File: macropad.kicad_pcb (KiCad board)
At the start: 2 copper layers, 78.5 x 59.5 mm, 47 parts, among them J1 DX07S016JA1R1500, SW1 SW_Push, SW10 SW_Push, SW2 SW_Push, SW3 SW_Push, SW5 SW_Push, SW6 SW_Push, SW7 SW_Push, SW8 SW_Push, SW9 SW_Push, U1 ATmega16U2-MU, Y1 16MHz

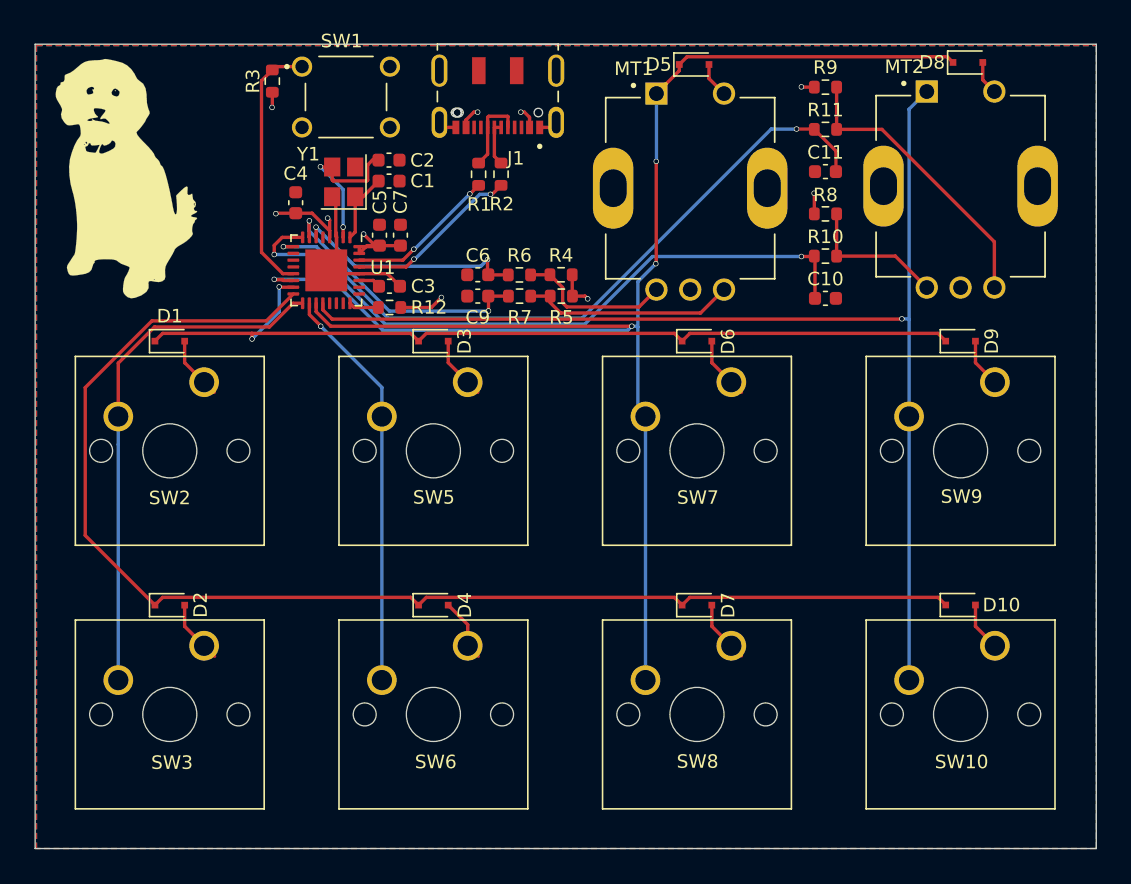
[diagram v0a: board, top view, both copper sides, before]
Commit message: Some aesthetic cleanup
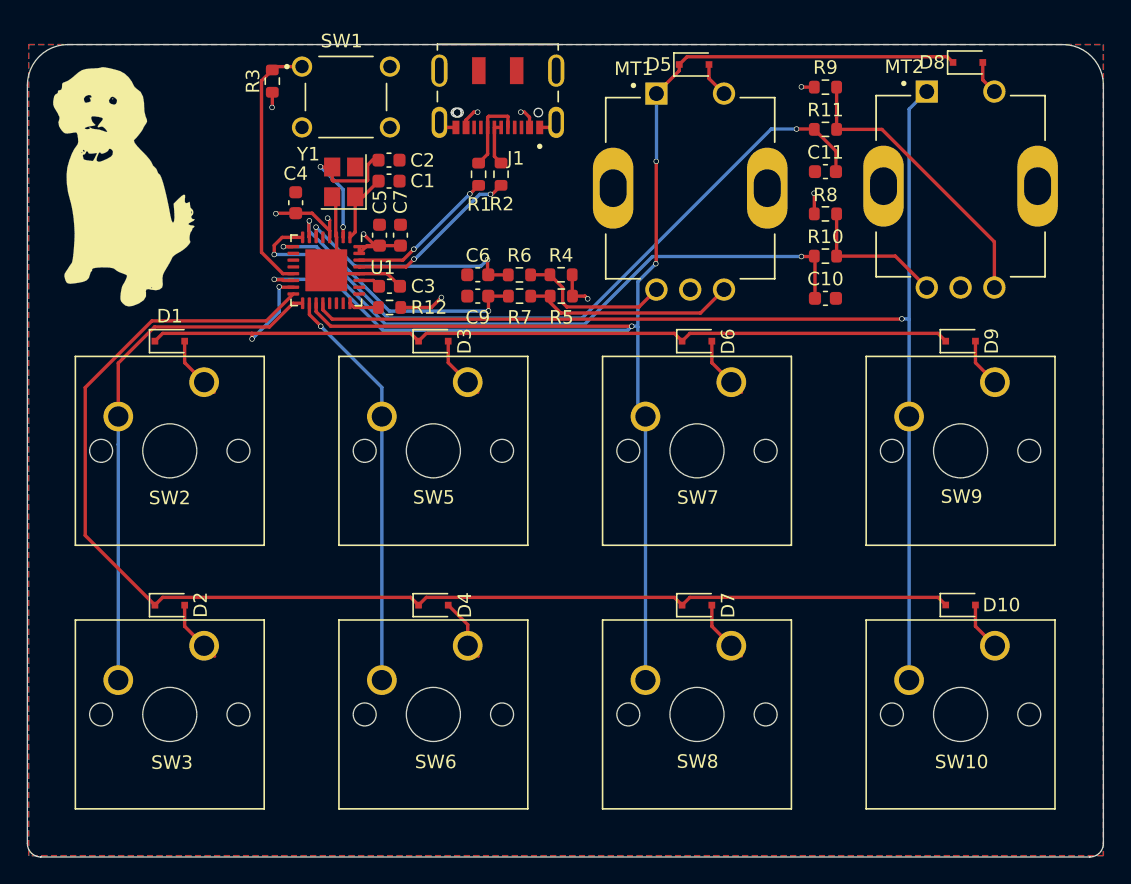
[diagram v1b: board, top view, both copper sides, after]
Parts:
- moved G*** 0.63 mm to (125.9, 67.5)
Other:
- board size 78.5 x 59.5 mm -> 79.6 x 60.1 mm
- board text added: "Eric Wood 3/21"
- board text added: "PB0-2 -> row0-2 PB3-6 -> col0-3 pd0-1 -> rotary 1 pd2-3 -> rotary 2"
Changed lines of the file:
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@@
   (general
     (thickness 1.6)
-    (drawings 4)
+    (drawings 10)
     (tracks 299)
     (zones 0)
@@
   )
   (module dsp_dev_board:frankie (layer F.Cu)
-    (at 126.065 66.925)
+    (at 125.875 67.5282)
     (fp_text reference G*** (at 0 0) (layer F.SilkS) hide
       (effects (font (size 1.524 1.524) (thickness 0.3)))
@@
     )
   )
-  (gr_line (start 198 56.5) (end 198 116) (layer Edge.Cuts) (width 0.1))
-  (gr_line (start 119.5 56.5) (end 198 56.5) (layer Edge.Cuts) (width 0.1))
-  (gr_line (start 119.5 116) (end 119.5 56.5) (layer Edge.Cuts) (width 0.1))
-  (gr_line (start 198 116) (end 119.5 116) (layer Edge.Cuts) (width 0.1))
+  (gr_text "PB0-2 -> row0-2\nPB3-6 -> col0-3\npd0-1 -> rotary 1\npd2-3 -> rotary 2" (at 160.175 93.825 180) (layer B.SilkS)
+    (effects (font (size 1 1) (thickness 0.15)) (justify mirror))
+  )
+  (gr_text "Eric Wood 3/21" (at 120.875 88.475 90) (layer B.SilkS)
+    (effects (font (size 1.5 1.5) (thickness 0.3)) (justify mirror))
+  )
+  (gr_line (start 118.925 115.625) (end 118.925 59.525) (layer Edge.Cuts) (width 0.05))
+  (gr_arc (start 121.925 59.525) (end 121.925 56.525) (angle -90) (layer Edge.Cuts) (width 0.05))
+  (gr_arc (start 195.525 59.525) (end 198.525 59.525) (angle -90) (layer Edge.Cuts) (width 0.05))
+  (gr_arc (start 197.525 115.625) (end 197.525 116.625) (angle -90) (layer Edge.Cuts) (width 0.05))
+  (gr_arc (start 119.925 115.625) (end 118.925 115.625) (angle -90) (layer Edge.Cuts) (width 0.05))
+  (gr_line (start 195.525 56.525) (end 121.925 56.525) (layer Edge.Cuts) (width 0.05))
+  (gr_line (start 198.525 115.625) (end 198.525 59.525) (layer Edge.Cuts) (width 0.05))
+  (gr_line (start 119.925 116.625) (end 197.525 116.625) (layer Edge.Cuts) (width 0.05))
   (segment (start 140.92501 74.50001) (end 140.725 74.3) (width 0.25) (layer F.Cu) (net 1) (status 30))
   (segment (start 141.2875 73.475) (end 141.0375 73.225) (width 0.25) (layer F.Cu) (net 1) (status 30))
@@
     (polygon
       (pts
-        (xy 198 116) (xy 119.6 116) (xy 119.6 56.6) (xy 198 56.6)
+        (xy 198.525 116.525) (xy 119.025 116.525) (xy 119.025 56.525) (xy 198.525 56.525)
       )
     )
@@
     (polygon
       (pts
-        (xy 198 116) (xy 119.6 116) (xy 119.6 56.6) (xy 198 56.6)
+        (xy 198.525 116.525) (xy 119.025 116.525) (xy 119.025 56.525) (xy 198.525 56.525)
       )
     )
